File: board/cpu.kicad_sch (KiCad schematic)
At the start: 10 parts, among them U1 MC68000P

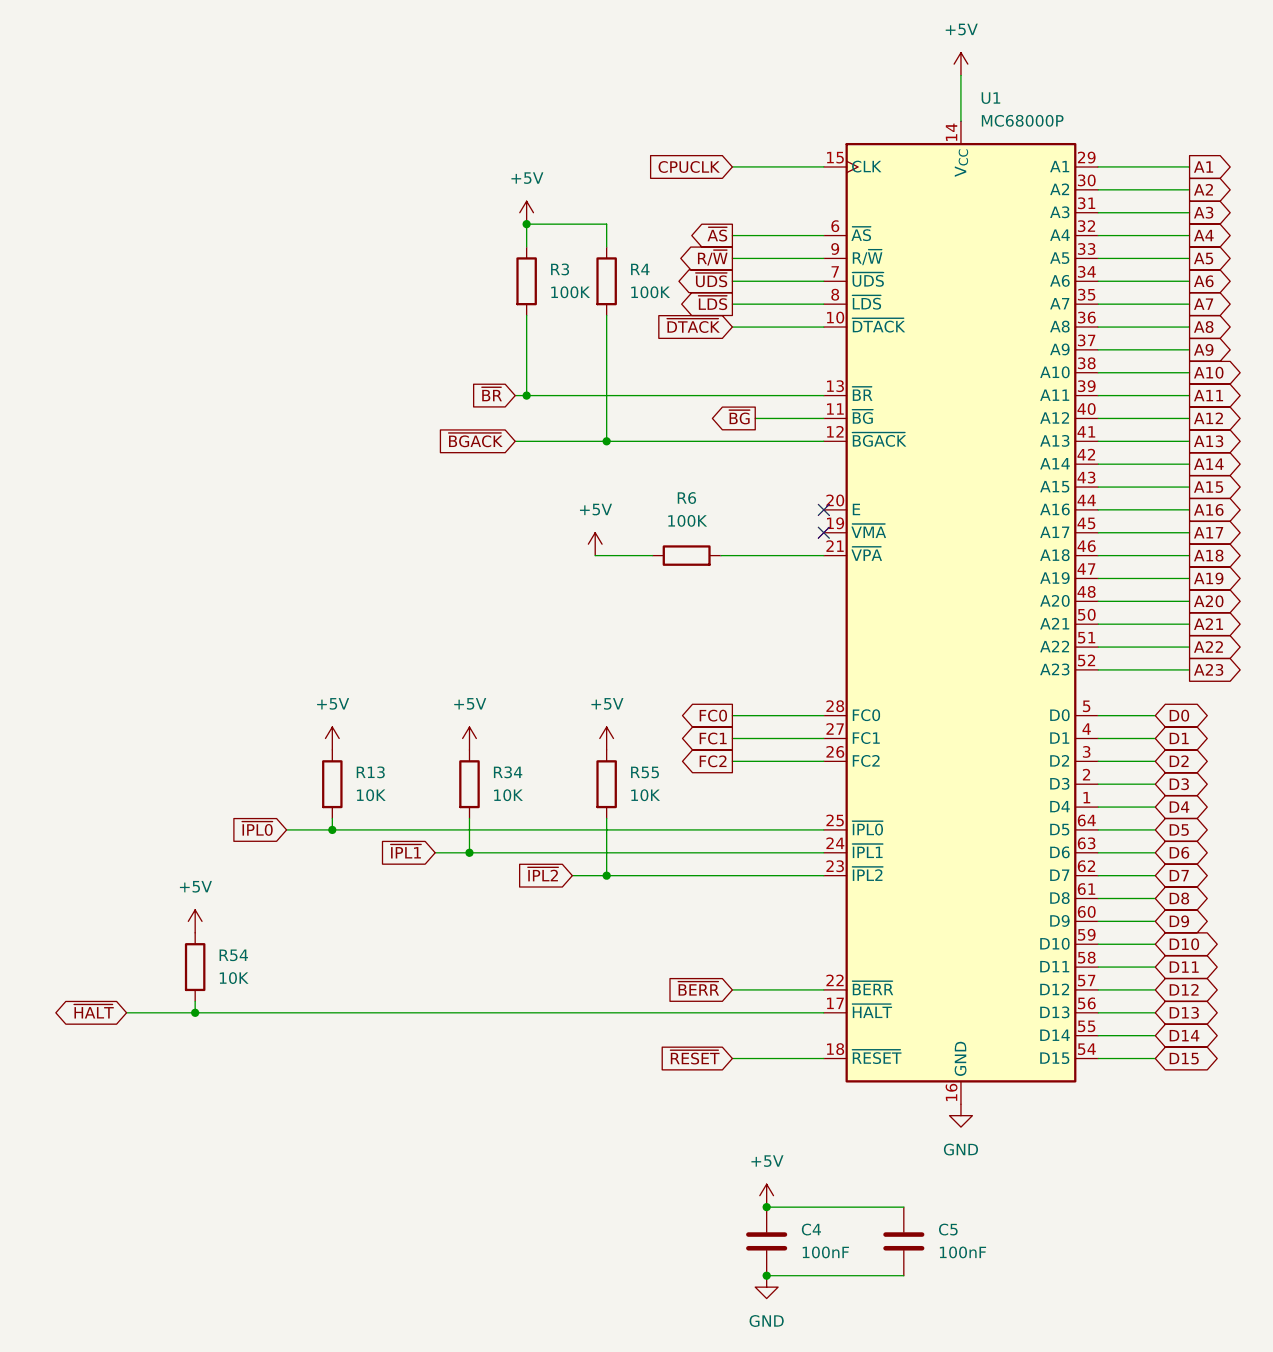
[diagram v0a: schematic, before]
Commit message: Board rev1 PCB complete, already have a spot fix
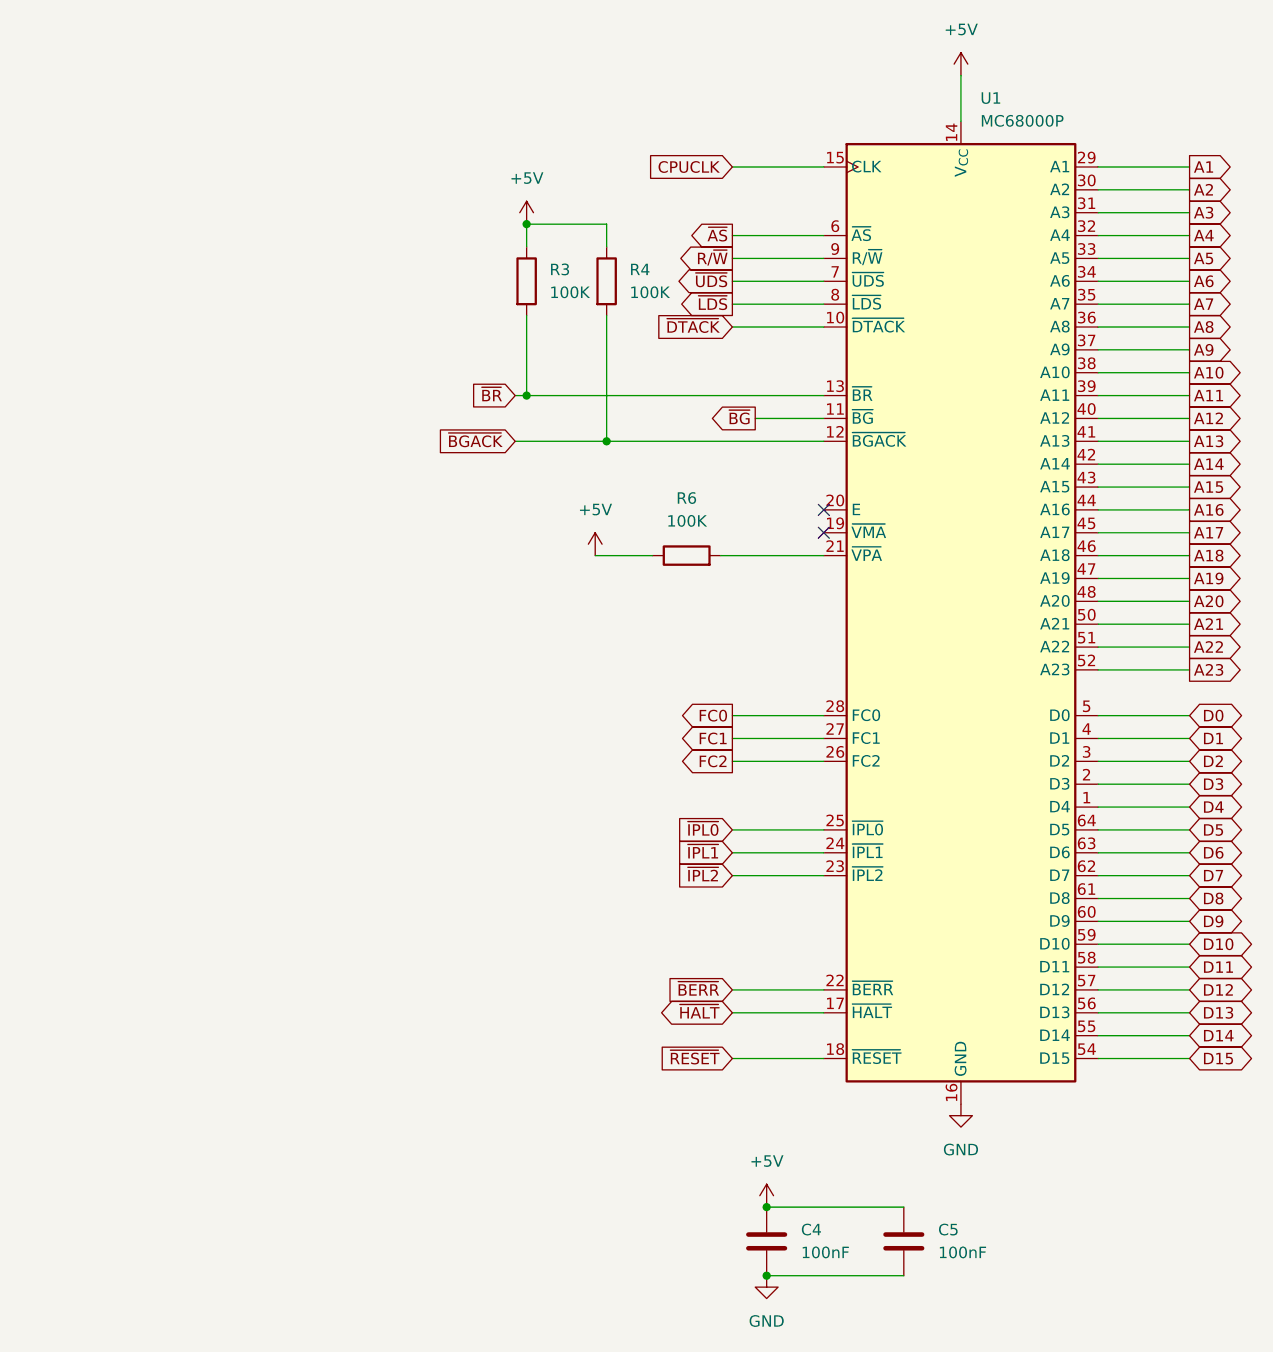
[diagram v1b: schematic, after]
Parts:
- removed R13, R34, R54, R55: 10K, Resistor_THT:R_Axial_DIN0207_L6.3mm_D2.5mm_P10.16mm_Horizontal, symbol Device:R
